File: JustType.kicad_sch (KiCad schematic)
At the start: 56 parts, among them J1 Conn_01x02, J2 Conn_01x02, SW1 SW_Push, SW10 SW_Push, SW11 SW_Push, SW12 SW_Push, SW13 SW_Push, SW14 SW_Push, SW15 SW_Push, SW16 SW_Push, SW17 SW_Push, SW18 SW_Push, SW19 SW_Push, SW19'1 SW_Push, SW2 SW_Push, SW20 SW_Push, SW21 SW_Push, SW22 SW_Push, SW23 SW_Push, SW24 SW_Push, SW25 SW_Push, SW3 SW_Push, SW4 SW_Push, SW5 SW_Push, SW6 SW_Push, SW7 SW_Push, SW8 SW_Push, SW9 SW_Push, U1 ProMicro

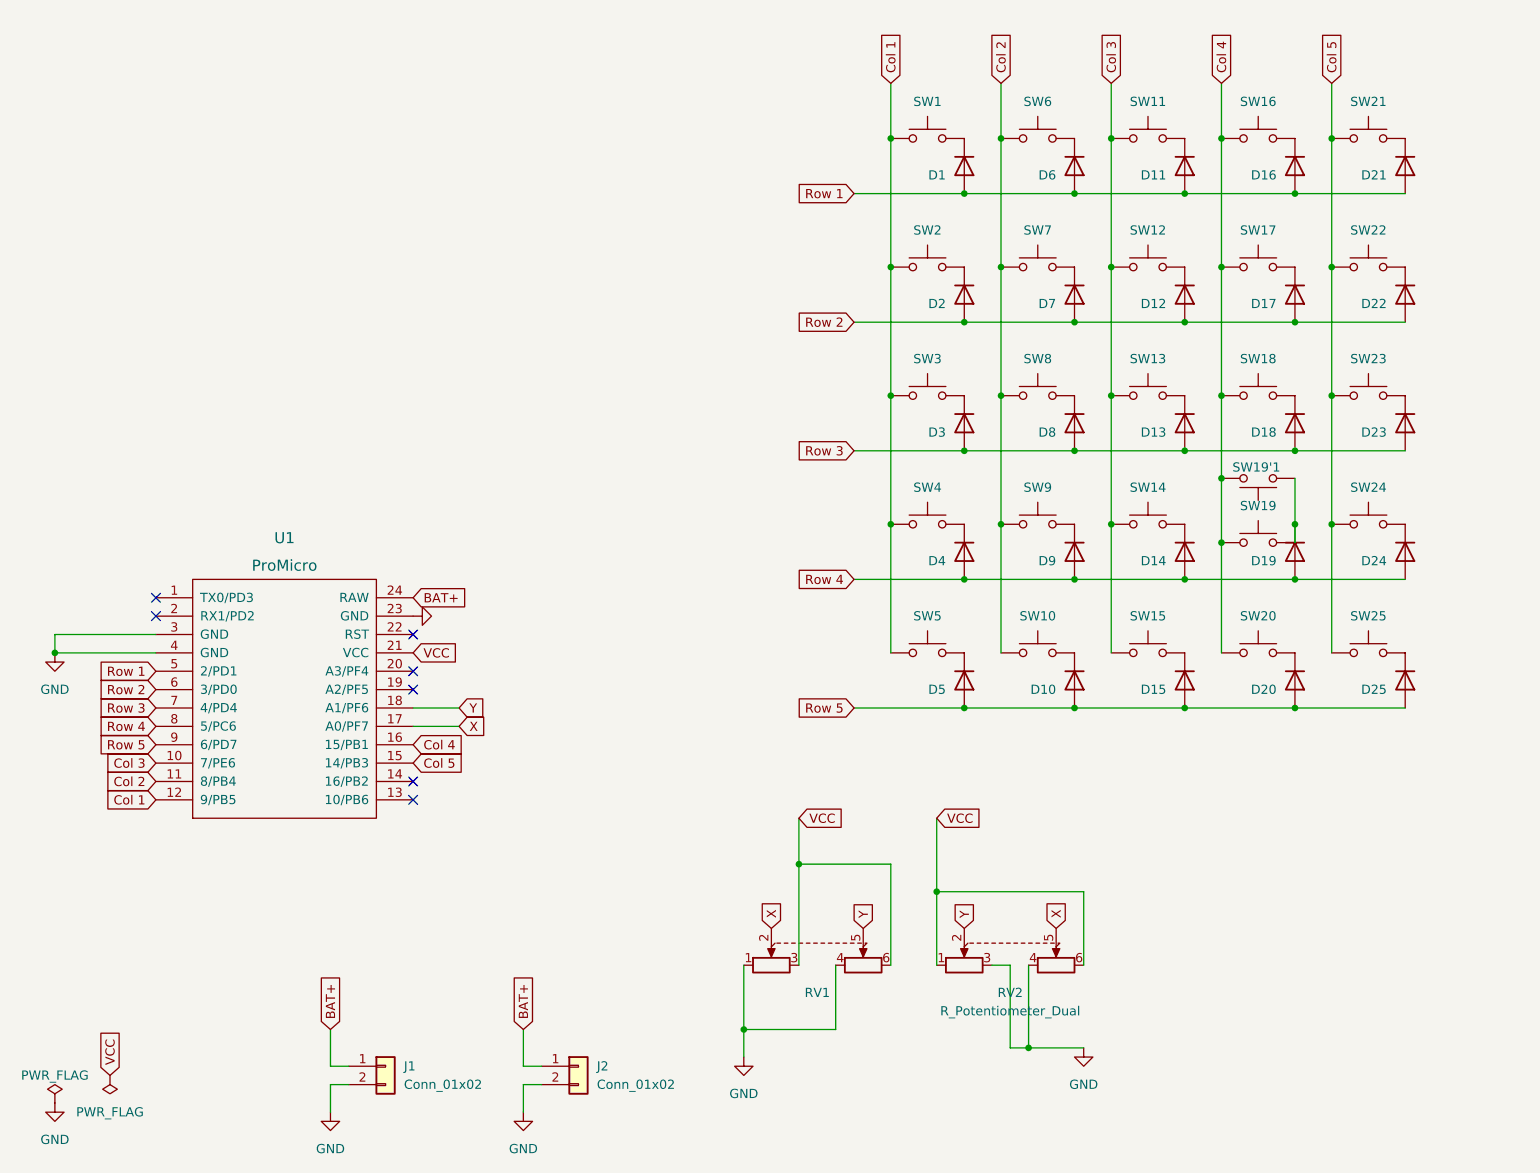
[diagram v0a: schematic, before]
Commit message: v4
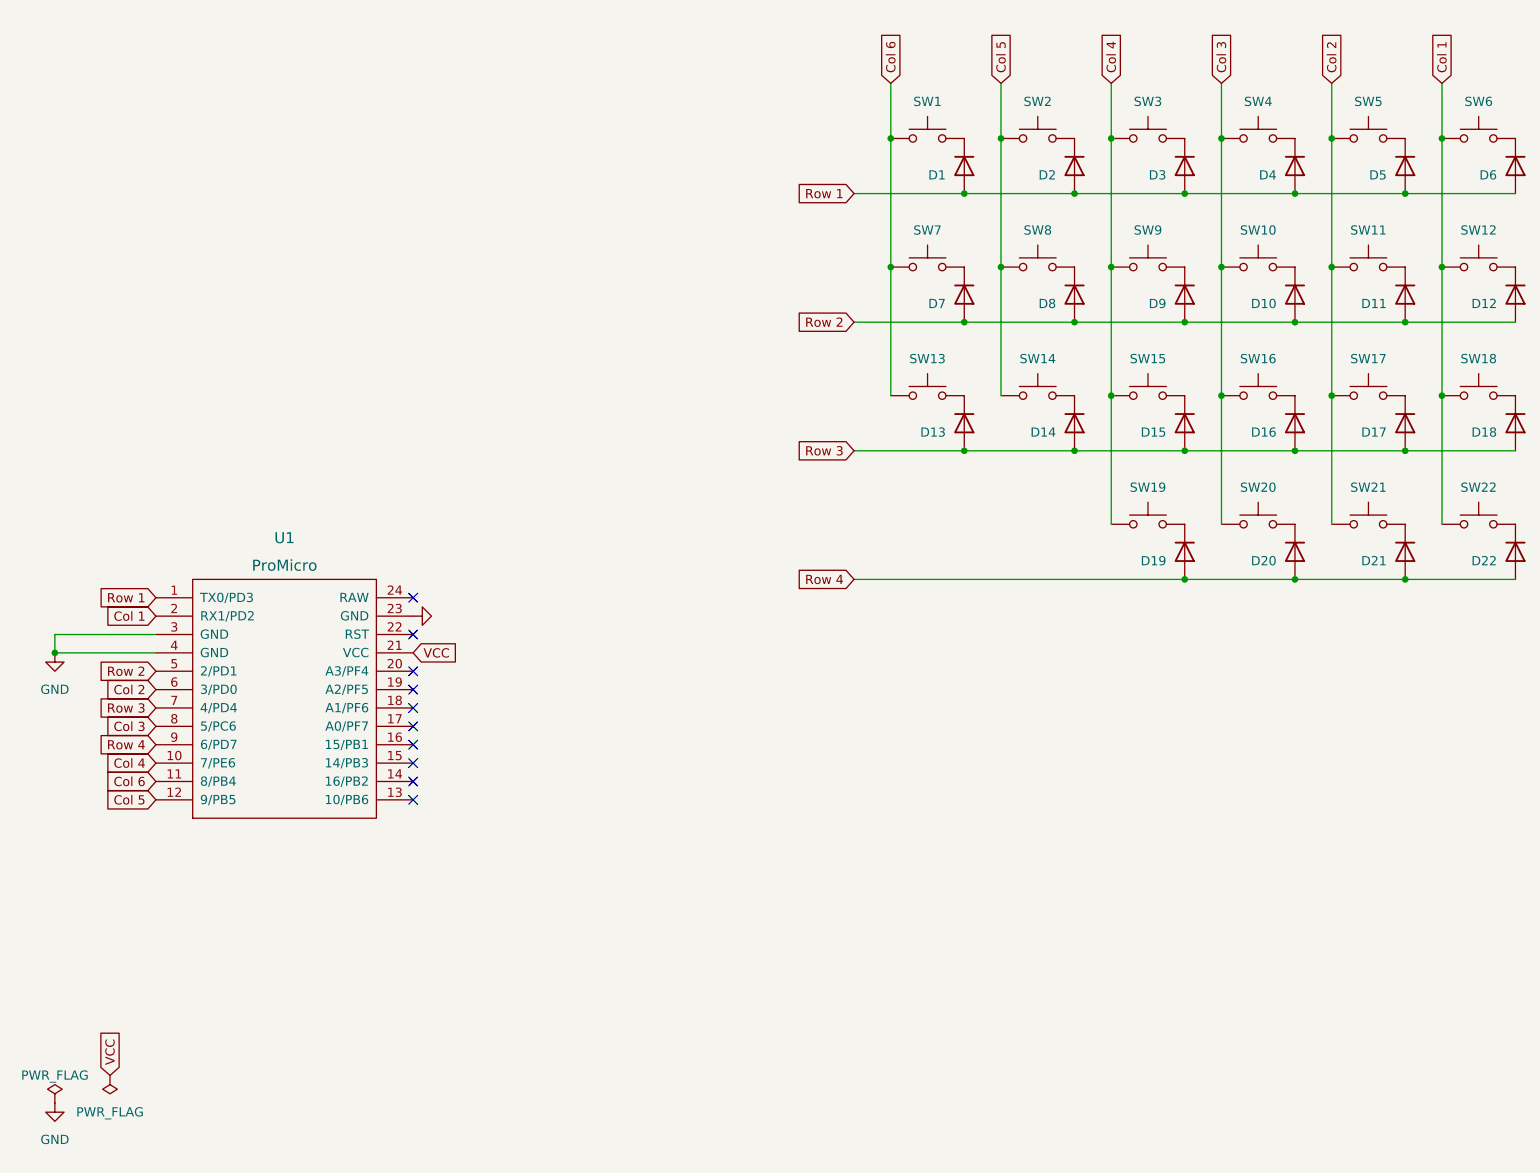
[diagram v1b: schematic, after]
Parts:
- removed D10, D15, D20, D25, D4, D5, D9: 1N4448W, Diode_SMD:D_SOD-123, symbol Diode:1N4448W
- removed J1, J2: Conn_01x02, Connector_JST:JST_PH_S2B-PH-K_1x02_P2.00mm_Horizontal, symbol Connector_Generic:Conn_01x02
- removed RV1, RV2: R_Potentiometer_Dual, keyboard_jsa:PSP thumbstick, symbol Device:R_Potentiometer_Dual
- removed SW10, SW15, SW19'1, SW20, SW25, SW4, SW5, SW9: SW_Push, keyboard_jsa:ChocV1_Hotswap, symbol Switch:SW_Push
- added D12, D18, D22, D6: 1N4448W, keyboard_jsa:D3_SMD_v2, symbol Diode:1N4448W
- added SW12, SW18, SW22, SW6: SW_Push, keyboard_jsa:ChocV1_Solder, symbol Switch:SW_Push
- D1: footprint Diode_SMD:D_SOD-123 -> keyboard_jsa:D3_SMD_v2
- D10: renamed from D17; footprint Diode_SMD:D_SOD-123 -> keyboard_jsa:D3_SMD_v2
- D11: renamed from D22; footprint Diode_SMD:D_SOD-123 -> keyboard_jsa:D3_SMD_v2
- D13: renamed from D3; footprint Diode_SMD:D_SOD-123 -> keyboard_jsa:D3_SMD_v2
- D14: renamed from D8; footprint Diode_SMD:D_SOD-123 -> keyboard_jsa:D3_SMD_v2
- D15: renamed from D13; footprint Diode_SMD:D_SOD-123 -> keyboard_jsa:D3_SMD_v2
- D16: renamed from D18; footprint Diode_SMD:D_SOD-123 -> keyboard_jsa:D3_SMD_v2
- D17: renamed from D23; footprint Diode_SMD:D_SOD-123 -> keyboard_jsa:D3_SMD_v2
- D19: renamed from D14; footprint Diode_SMD:D_SOD-123 -> keyboard_jsa:D3_SMD_v2
- D2: renamed from D6; footprint Diode_SMD:D_SOD-123 -> keyboard_jsa:D3_SMD_v2
- D20: renamed from D19; footprint Diode_SMD:D_SOD-123 -> keyboard_jsa:D3_SMD_v2
- D21: renamed from D24; footprint Diode_SMD:D_SOD-123 -> keyboard_jsa:D3_SMD_v2
- D3: renamed from D11; footprint Diode_SMD:D_SOD-123 -> keyboard_jsa:D3_SMD_v2
- D4: renamed from D16; footprint Diode_SMD:D_SOD-123 -> keyboard_jsa:D3_SMD_v2
- D5: renamed from D21; footprint Diode_SMD:D_SOD-123 -> keyboard_jsa:D3_SMD_v2
- D7: renamed from D2; footprint Diode_SMD:D_SOD-123 -> keyboard_jsa:D3_SMD_v2
- D8: renamed from D7; footprint Diode_SMD:D_SOD-123 -> keyboard_jsa:D3_SMD_v2
- D9: renamed from D12; footprint Diode_SMD:D_SOD-123 -> keyboard_jsa:D3_SMD_v2
- SW1: footprint keyboard_jsa:ChocV1_Hotswap -> keyboard_jsa:ChocV1_Solder
- SW10: renamed from SW17; footprint keyboard_jsa:ChocV1_Hotswap -> keyboard_jsa:ChocV1_Solder
- SW11: renamed from SW22; footprint keyboard_jsa:ChocV1_Hotswap -> keyboard_jsa:ChocV1_Solder
- SW13: renamed from SW3; footprint keyboard_jsa:ChocV1_Hotswap -> keyboard_jsa:ChocV1_Solder
- SW14: renamed from SW8; footprint keyboard_jsa:ChocV1_Hotswap -> keyboard_jsa:ChocV1_Solder
- SW15: renamed from SW13; footprint keyboard_jsa:ChocV1_Hotswap -> keyboard_jsa:ChocV1_Solder
- SW16: renamed from SW18; footprint keyboard_jsa:ChocV1_Hotswap -> keyboard_jsa:ChocV1_Solder
- SW17: renamed from SW23; footprint keyboard_jsa:ChocV1_Hotswap -> keyboard_jsa:ChocV1_Solder
- SW19: renamed from SW14; footprint keyboard_jsa:ChocV1_Hotswap -> keyboard_jsa:ChocV1_Solder
- SW2: renamed from SW6; footprint keyboard_jsa:ChocV1_Hotswap -> keyboard_jsa:ChocV1_Solder
- SW20: renamed from SW19; footprint keyboard_jsa:ChocV1_Hotswap -> keyboard_jsa:ChocV1_Solder
- SW21: renamed from SW24; footprint keyboard_jsa:ChocV1_Hotswap -> keyboard_jsa:ChocV1_Solder
- SW3: renamed from SW11; footprint keyboard_jsa:ChocV1_Hotswap -> keyboard_jsa:ChocV1_Solder
- SW4: renamed from SW16; footprint keyboard_jsa:ChocV1_Hotswap -> keyboard_jsa:ChocV1_Solder
- SW5: renamed from SW21; footprint keyboard_jsa:ChocV1_Hotswap -> keyboard_jsa:ChocV1_Solder
- SW7: renamed from SW2; footprint keyboard_jsa:ChocV1_Hotswap -> keyboard_jsa:ChocV1_Solder
- SW8: renamed from SW7; footprint keyboard_jsa:ChocV1_Hotswap -> keyboard_jsa:ChocV1_Solder
- SW9: renamed from SW12; footprint keyboard_jsa:ChocV1_Hotswap -> keyboard_jsa:ChocV1_Solder
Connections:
- net Row 5 is gone; now on net Row 4: U1.9 (6/PD7)
- net Col 1: now also U1.2 (RX1/PD2), SW12.1, SW18.1, SW22.1, SW6.1; no longer SW1.1, SW13.1, SW7.1, U1.12 (9/PB5)
- net Col 2: now also SW11.1, SW17.1, SW21.1, SW5.1, U1.6 (3/PD0); no longer SW14.1, SW2.1, SW8.1, U1.11 (8/PB4)
- net Col 3: now also SW10.1, SW16.1, SW20.1, SW4.1, U1.8 (5/PC6); no longer SW15.1, SW19.1, SW3.1, SW9.1, U1.10 (7/PE6)
- net Col 4: now also SW15.1, SW19.1, SW3.1, SW9.1, U1.10 (7/PE6); no longer SW10.1, SW16.1, SW20.1, SW4.1, U1.16 (15/PB1)
- net Col 5: now also SW14.1, SW2.1, SW8.1, U1.12 (9/PB5); no longer SW11.1, SW17.1, SW21.1, SW5.1, U1.15 (14/PB3)
- net Row 1: now also U1.1 (TX0/PD3), D6.2 (A); no longer U1.5 (2/PD1)
- net Row 2: now also U1.5 (2/PD1), D12.2 (A); no longer U1.6 (3/PD0)
- net Row 3: now also D18.2 (A)
- net Row 4: now also D22.2 (A); no longer U1.8 (5/PC6)
- net BAT+: no longer names the net of U1.24 (RAW)
- net X: no longer names the net of U1.17 (A0/PF7)
- net Y: no longer names the net of U1.18 (A1/PF6)
- new net: D18.1 (K), SW18.2
- new net: D12.1 (K), SW12.2
- new net: D22.1 (K), SW22.2
- new net: D6.1 (K), SW6.2
- new net Col 6: SW1.1, SW13.1, SW7.1, U1.11 (8/PB4)
- no-connect marks 7 -> 10
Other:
- moved on the sheet: SW20
